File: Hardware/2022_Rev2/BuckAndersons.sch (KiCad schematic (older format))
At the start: 18 parts, among them U3 OKI-78SR-5_1.5-W36-C, U4 OKI-78SR-5_1.5-W36-C

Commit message: Finished footprint signatures and started schematic
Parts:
- Conn13, Conn15, Conn16: footprint (none) -> MRDT_Connectors:Anderson_3_Vertical_Side_by_Side
- Conn14, Conn17, Conn18: footprint (none) -> MRDT_Connectors:Anderson_2_Vertical_Sidy_by_Side
- R3, R4: footprint (none) -> Resistor_SMD:R_0603_1608Metric_Pad0.98x0.95mm_HandSolder
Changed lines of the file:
@@
 F 0 "Conn15" H 4908 1787 60  0000 C CNN
 F 1 "Aux_1_Out" H 4908 1681 60  0000 C CNN
-F 2 "" H 4550 850 60  0001 C CNN
+F 2 "MRDT_Connectors:Anderson_3_Vertical_Side_by_Side" H 4550 850 60  0001 C CNN
 F 3 "" H 4550 850 60  0001 C CNN
 	4    4700 1400
@@
 F 0 "Conn15" H 4908 2287 60  0000 C CNN
 F 1 "Aux_1_Out" H 4908 2181 60  0000 C CNN
-F 2 "" H 4550 1350 60  0001 C CNN
+F 2 "MRDT_Connectors:Anderson_3_Vertical_Side_by_Side" H 4550 1350 60  0001 C CNN
 F 3 "" H 4550 1350 60  0001 C CNN
 	2    4700 1900
@@
 F 0 "Conn15" H 4908 2787 60  0000 C CNN
 F 1 "Aux_1_Out" H 4908 2681 60  0000 C CNN
-F 2 "" H 4550 1850 60  0001 C CNN
+F 2 "MRDT_Connectors:Anderson_3_Vertical_Side_by_Side" H 4550 1850 60  0001 C CNN
 F 3 "" H 4550 1850 60  0001 C CNN
 	1    4700 2400
@@
 F 0 "Conn16" H 4908 3887 60  0000 C CNN
 F 1 "Aux_2_Out" H 4908 3781 60  0000 C CNN
-F 2 "" H 4550 2950 60  0001 C CNN
+F 2 "MRDT_Connectors:Anderson_3_Vertical_Side_by_Side" H 4550 2950 60  0001 C CNN
 F 3 "" H 4550 2950 60  0001 C CNN
 	4    4700 3500
@@
 F 0 "Conn16" H 4908 4387 60  0000 C CNN
 F 1 "Aux_2_Out" H 4908 4281 60  0000 C CNN
-F 2 "" H 4550 3450 60  0001 C CNN
+F 2 "MRDT_Connectors:Anderson_3_Vertical_Side_by_Side" H 4550 3450 60  0001 C CNN
 F 3 "" H 4550 3450 60  0001 C CNN
 	2    4700 4000
@@
 F 0 "Conn16" H 4908 4887 60  0000 C CNN
 F 1 "Aux_2_Out" H 4908 4781 60  0000 C CNN
-F 2 "" H 4550 3950 60  0001 C CNN
+F 2 "MRDT_Connectors:Anderson_3_Vertical_Side_by_Side" H 4550 3950 60  0001 C CNN
 F 3 "" H 4550 3950 60  0001 C CNN
 	1    4700 4500
@@
 F 0 "Conn17" H 6408 1787 60  0000 C CNN
 F 1 "Aux_1_In" H 6408 1681 60  0000 C CNN
-F 2 "" H 6050 850 60  0001 C CNN
+F 2 "MRDT_Connectors:Anderson_2_Vertical_Sidy_by_Side" H 6050 850 60  0001 C CNN
 F 3 "" H 6050 850 60  0001 C CNN
 	3    6200 1400
@@
 F 0 "Conn17" H 6408 2287 60  0000 C CNN
 F 1 "Aux_1_In" H 6408 2181 60  0000 C CNN
-F 2 "" H 6050 1350 60  0001 C CNN
+F 2 "MRDT_Connectors:Anderson_2_Vertical_Sidy_by_Side" H 6050 1350 60  0001 C CNN
 F 3 "" H 6050 1350 60  0001 C CNN
 	1    6200 1900
@@
 F 0 "Conn18" H 6408 3887 60  0000 C CNN
 F 1 "Aux_2_In" H 6408 3781 60  0000 C CNN
-F 2 "" H 6050 2950 60  0001 C CNN
+F 2 "MRDT_Connectors:Anderson_2_Vertical_Sidy_by_Side" H 6050 2950 60  0001 C CNN
 F 3 "" H 6050 2950 60  0001 C CNN
 	3    6200 3500
@@
 F 0 "Conn18" H 6408 4387 60  0000 C CNN
 F 1 "Aux_2_In" H 6408 4281 60  0000 C CNN
-F 2 "" H 6050 3450 60  0001 C CNN
+F 2 "MRDT_Connectors:Anderson_2_Vertical_Sidy_by_Side" H 6050 3450 60  0001 C CNN
 F 3 "" H 6050 3450 60  0001 C CNN
 	1    6200 4000
@@
 F 0 "Conn13" H 1608 6037 60  0000 C CNN
 F 1 "Aux_GP_Out" H 1608 5931 60  0000 C CNN
-F 2 "" H 1250 5100 60  0001 C CNN
+F 2 "MRDT_Connectors:Anderson_3_Vertical_Side_by_Side" H 1250 5100 60  0001 C CNN
 F 3 "" H 1250 5100 60  0001 C CNN
 	4    1400 5650
@@
 F 0 "Conn13" H 1608 6537 60  0000 C CNN
 F 1 "Aux_GP_Out" H 1608 6431 60  0000 C CNN
-F 2 "" H 1250 5600 60  0001 C CNN
+F 2 "MRDT_Connectors:Anderson_3_Vertical_Side_by_Side" H 1250 5600 60  0001 C CNN
 F 3 "" H 1250 5600 60  0001 C CNN
 	2    1400 6150
@@
 F 0 "Conn13" H 1608 7037 60  0000 C CNN
 F 1 "Aux_GP_Out" H 1608 6931 60  0000 C CNN
-F 2 "" H 1250 6100 60  0001 C CNN
+F 2 "MRDT_Connectors:Anderson_3_Vertical_Side_by_Side" H 1250 6100 60  0001 C CNN
 F 3 "" H 1250 6100 60  0001 C CNN
 	1    1400 6650
@@
 F 0 "Conn14" H 3108 6037 60  0000 C CNN
 F 1 "Aux_GP_In" H 3108 5931 60  0000 C CNN
-F 2 "" H 2750 5100 60  0001 C CNN
+F 2 "MRDT_Connectors:Anderson_2_Vertical_Sidy_by_Side" H 2750 5100 60  0001 C CNN
 F 3 "" H 2750 5100 60  0001 C CNN
 	3    2900 5650
@@
 F 0 "Conn14" H 3108 6537 60  0000 C CNN
 F 1 "Aux_GP_In" H 3108 6431 60  0000 C CNN
-F 2 "" H 2750 5600 60  0001 C CNN
+F 2 "MRDT_Connectors:Anderson_2_Vertical_Sidy_by_Side" H 2750 5600 60  0001 C CNN
 F 3 "" H 2750 5600 60  0001 C CNN
 	1    2900 6150
@@
 F 0 "R3" V 3043 1400 50  0000 C CNN
 F 1 "510" V 3134 1400 50  0000 C CNN
-F 2 "" V 3180 1400 50  0001 C CNN
+F 2 "Resistor_SMD:R_0603_1608Metric_Pad0.98x0.95mm_HandSolder" V 3180 1400 50  0001 C CNN
 F 3 "~" H 3250 1400 50  0001 C CNN
 	1    3250 1400
@@
 F 0 "R4" V 3043 3000 50  0000 C CNN
 F 1 "510" V 3134 3000 50  0000 C CNN
-F 2 "" V 3180 3000 50  0001 C CNN
+F 2 "Resistor_SMD:R_0603_1608Metric_Pad0.98x0.95mm_HandSolder" V 3180 3000 50  0001 C CNN
 F 3 "~" H 3250 3000 50  0001 C CNN
 	1    3250 3000

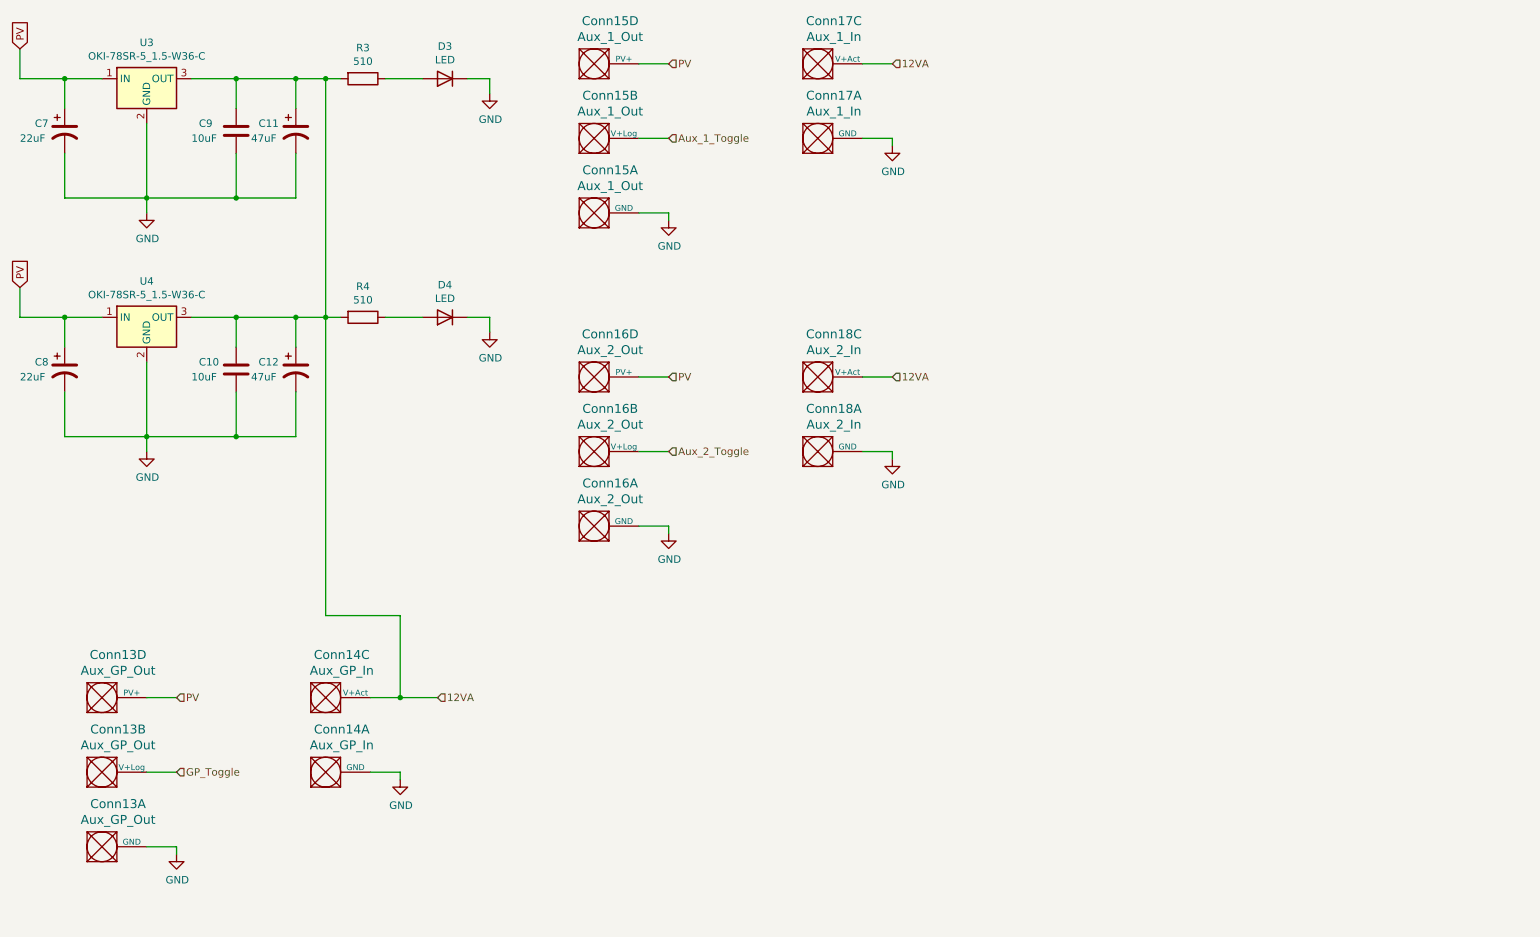
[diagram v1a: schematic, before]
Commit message: Lots of Changes
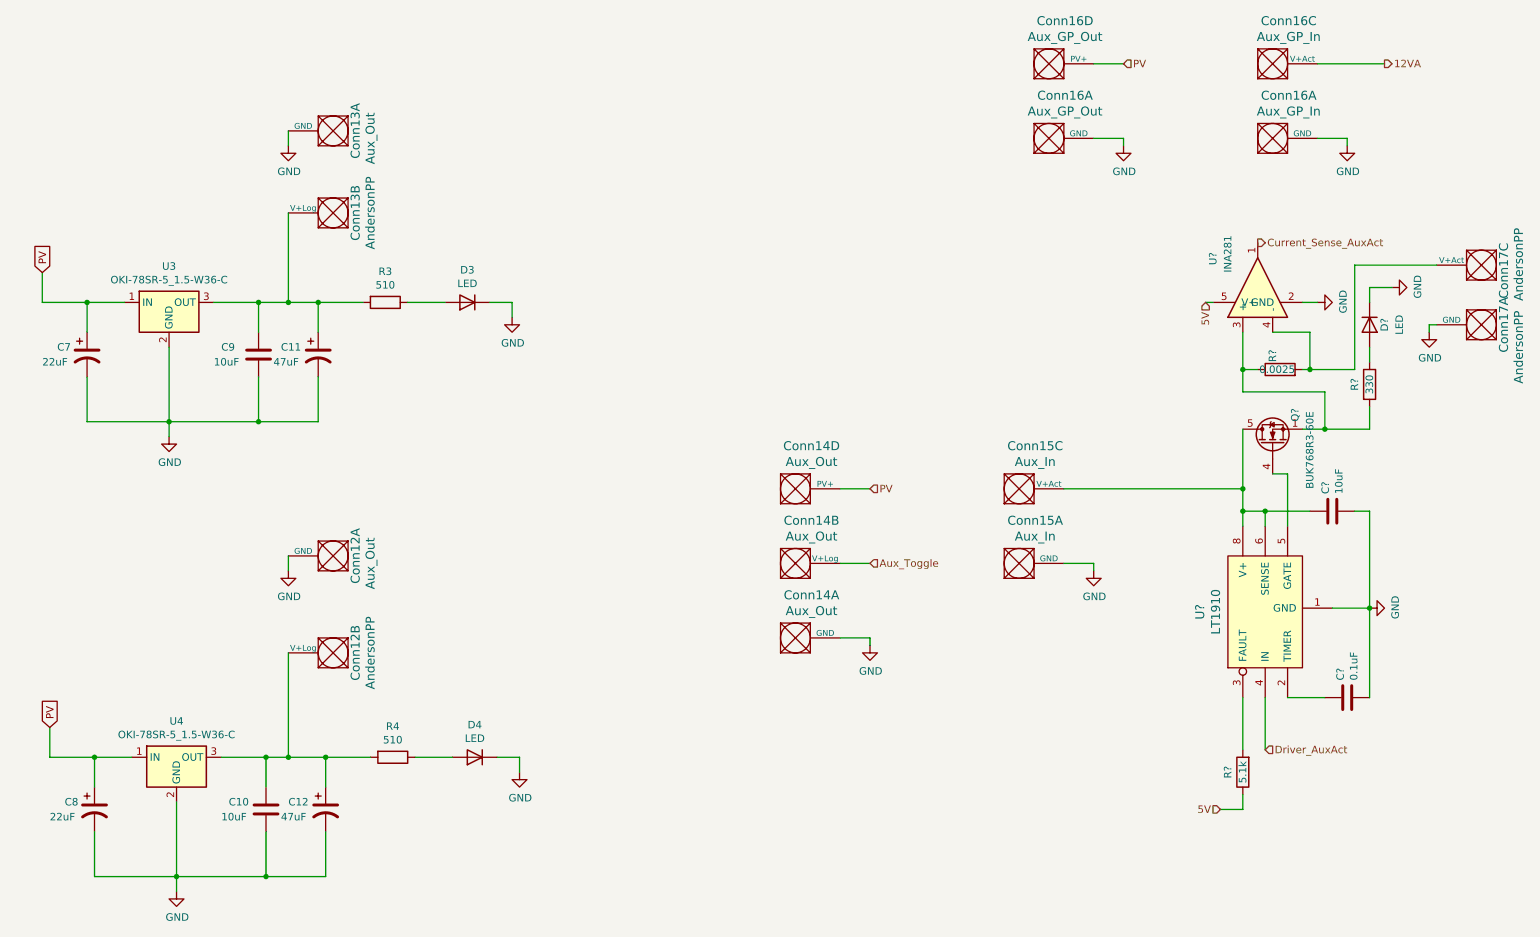
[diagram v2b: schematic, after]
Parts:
- removed unit 2 of Conn13
- removed Conn16: Aux_2_Out, MRDT_Connectors:Anderson_3_Vertical_Side_by_Side, symbol 2022_Rev2-rescue:AndersonPP-MRDT_Connectors
- removed Conn18: Aux_2_In, MRDT_Connectors:Anderson_2_Vertical_Sidy_by_Side, symbol 2022_Rev2-rescue:AndersonPP-MRDT_Connectors
- added C?: 0.1uF, Capacitor_SMD:C_0603_1608Metric_Pad1.08x0.95mm_HandSolder, symbol Device:C
- added C?: 10uF, Capacitor_SMD:C_0603_1608Metric_Pad1.08x0.95mm_HandSolder, symbol Device:C
- added Conn12, Conn13: AndersonPP, MRDT_Connectors:Anderson_2_Vertical_Sidy_by_Side, symbol MRDT_Connectors:AndersonPP
- added Conn17: AndersonPP, MRDT_Connectors:Anderson_2_Vertical_Side_by_Side_PV, symbol 2022_Rev2-rescue:AndersonPP-MRDT_Connectors
- added D?: LED, Diode_SMD:D_0603_1608Metric_Pad1.05x0.95mm_HandSolder, symbol Device:D
- added Q?: BUK768R3-60E, Package_TO_SOT_SMD:LFPAK33, symbol Transistor_FET:BUK7M9R9-60EX
- added R?: 5.1k, Resistor_SMD:R_0603_1608Metric_Pad0.98x0.95mm_HandSolder, symbol Device:R
- added R?: 330, Resistor_SMD:R_0603_1608Metric_Pad0.98x0.95mm_HandSolder, symbol Device:R
- added R?: 0.0025, Resistor_SMD:R_2512_6332Metric_Pad1.40x3.35mm_HandSolder, symbol Device:R
- added U?: LT1910, Package_SO:SOIC-8_3.9x4.9mm_P1.27mm, symbol 2022_Rev2-rescue:LT1910-MRDT_ICs
- added U?: INA281, Package_TO_SOT_SMD:SOT-23-5, symbol 2022_Rev2-rescue:INA281-MRDT_ICs
- Conn14: renamed from Conn15; value Aux_1_Out -> Aux_Out
- Conn15: renamed from Conn17; value Aux_1_In -> Aux_In
- renumbered Conn13 to Conn16, Conn14 to Conn16
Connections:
- net 12VA: no longer C10.1, C11.1, C12.1, C9.1, Conn15.3 (V+Act), R3.2, R4.2, U3.3 (OUT), U4.3 (OUT)
- net GND: now also C?.2, C?.2, Conn12.1 (GND), Conn13.1 (GND), Conn17.1 (GND), D?.1 (K), U?.1 (GND), U?.2 (GND)
- net Aux_1_Toggle renamed Aux_Toggle
- new net: C?.1, Conn15.3 (V+Act), Q?.5 (D), U?.6 (SENSE), U?.8 (V+)
- new net: C11.1, C9.1, Conn13.2 (V+Log), R3.2, U3.3 (OUT)
- new net: C10.1, C12.1, Conn12.2 (V+Log), R4.2, U4.3 (OUT)
- new net: R?.2, U?.3 (FAULT)
- new net: C?.1, U?.2 (TIMER)
- new net: Q?.4 (G), U?.5 (GATE)
- new net: Q?.1 (S), Q?.2 (S), Q?.3 (S), R?.1, R?.2, U?.3 (+)
- new net: D?.2 (A), R?.1
- new net: Conn17.3 (V+Act), R?.2, U?.4 (-)
- new net 5V: R?.1, U?.5 (V+)
- new net Current_Sense_AuxAct: U?.1
- new net Driver_AuxAct: U?.4 (IN)
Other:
- moved on the sheet: C10, C11, C12, C7, C8, C9, Conn14A, Conn14B, Conn14D, Conn15A, Conn15C, Conn16A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
